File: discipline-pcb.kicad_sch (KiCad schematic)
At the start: 143 parts, among them SW1 KEYSW, SW10 KEYSW, SW11 KEYSW, SW12 KEYSW, SW13 KEYSW, SW14 KEYSW, SW16 KEYSW, SW17 KEYSW, SW18 KEYSW, SW19 KEYSW, SW2 KEYSW, SW20 KEYSW, SW21 KEYSW, SW22 KEYSW, SW23 KEYSW, SW24 KEYSW, SW25 KEYSW, SW26 KEYSW, SW27 KEYSW, SW28 KEYSW, SW29 KEYSW, SW3 KEYSW, SW31 KEYSW, SW32 KEYSW, SW33 KEYSW, SW34 KEYSW, SW35 KEYSW, SW36 KEYSW, SW37 KEYSW, SW38 KEYSW, SW39 KEYSW, SW4 KEYSW, SW40 KEYSW, SW41 KEYSW, SW42 KEYSW, SW43 KEYSW, SW45 KEYSW, SW46 KEYSW, SW47 KEYSW, SW48 KEYSW, SW49 KEYSW, SW5 KEYSW, SW50 KEYSW, SW51 KEYSW, SW52 KEYSW, SW53 KEYSW, SW54 KEYSW, SW55 KEYSW, SW56 KEYSW, SW57 KEYSW, SW59 KEYSW, SW6 KEYSW, SW60 KEYSW, SW61 KEYSW, SW62 KEYSW, SW7 KEYSW, SW72 KEYSW, SW73 KEYSW, SW74 KEYSW, SW75 KEYSW, SW76 KEYSW, SW77 KEYSW, SW78 KEYSW, SW79 KEYSW, SW8 KEYSW, SW80 KEYSW, SW81 KEYSW, SW82 KEYSW, SW83 KEYSW, SW9 KEYSW

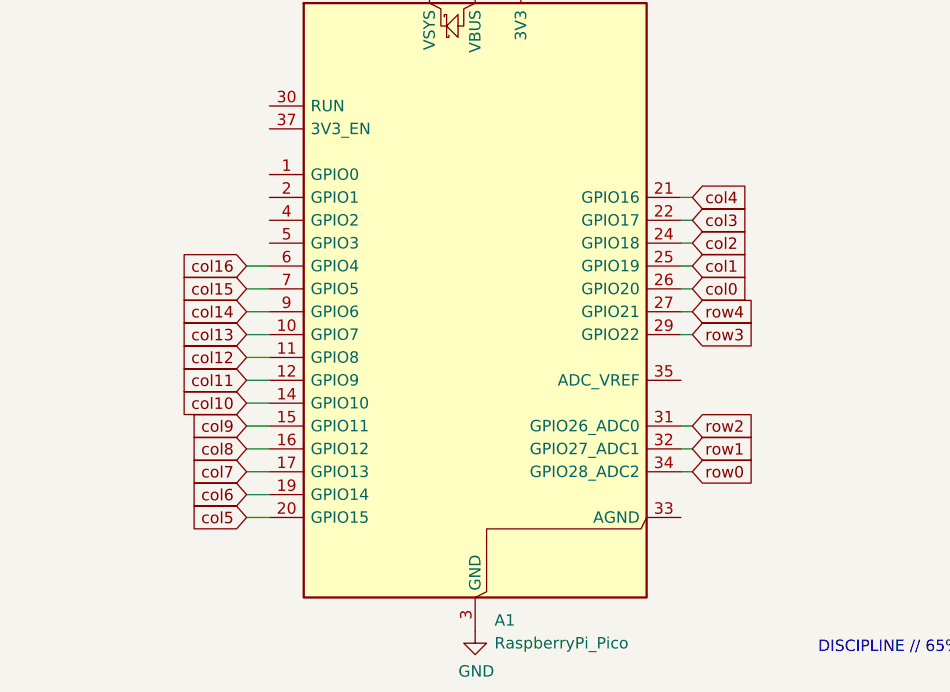
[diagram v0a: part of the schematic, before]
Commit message: add dru
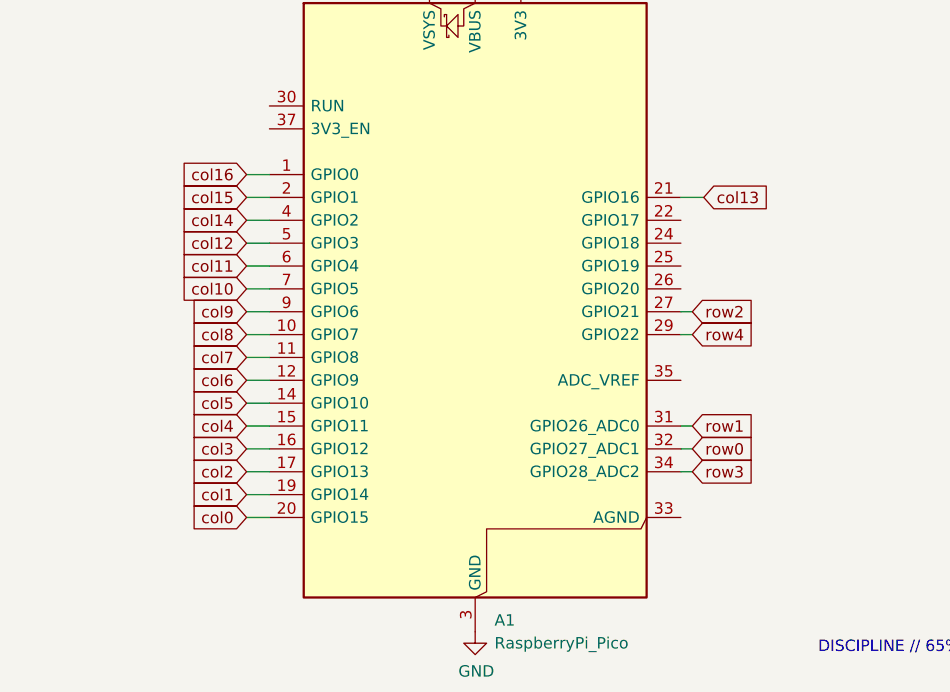
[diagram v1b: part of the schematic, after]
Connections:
- net col0: now also A1.20 (GPIO15); no longer A1.26 (GPIO20)
- net col1: now also A1.19 (GPIO14); no longer A1.25 (GPIO19)
- net col10: now also A1.7 (GPIO5); no longer A1.14 (GPIO10)
- net col11: now also A1.6 (GPIO4); no longer A1.12 (GPIO9)
- net col12: now also A1.5 (GPIO3); no longer A1.11 (GPIO8)
- net col13: now also A1.21 (GPIO16); no longer A1.10 (GPIO7)
- net col14: now also A1.4 (GPIO2); no longer A1.9 (GPIO6)
- net col15: now also A1.2 (GPIO1); no longer A1.7 (GPIO5)
- net col16: now also A1.1 (GPIO0); no longer A1.6 (GPIO4)
- net col2: now also A1.17 (GPIO13); no longer A1.24 (GPIO18)
- net col3: now also A1.16 (GPIO12); no longer A1.22 (GPIO17)
- net col4: now also A1.15 (GPIO11); no longer A1.21 (GPIO16)
- net col5: now also A1.14 (GPIO10); no longer A1.20 (GPIO15)
- net col6: now also A1.12 (GPIO9); no longer A1.19 (GPIO14)
- net col7: now also A1.11 (GPIO8); no longer A1.17 (GPIO13)
- net col8: now also A1.10 (GPIO7); no longer A1.16 (GPIO12)
- net col9: now also A1.9 (GPIO6); no longer A1.15 (GPIO11)
- net row0: now also A1.32 (GPIO27_ADC1); no longer A1.34 (GPIO28_ADC2)
- net row1: now also A1.31 (GPIO26_ADC0); no longer A1.32 (GPIO27_ADC1)
- net row2: now also A1.27 (GPIO21); no longer A1.31 (GPIO26_ADC0)
- net row3: now also A1.34 (GPIO28_ADC2); no longer A1.29 (GPIO22)
- net row4: now also A1.29 (GPIO22); no longer A1.27 (GPIO21)
